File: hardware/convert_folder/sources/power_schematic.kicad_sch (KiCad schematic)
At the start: 31 parts, among them CN1 5-146285-2, CN11 5-146285-2, CN13 4243-0, CN15 JST 2 position header 2.5mm, CN2 4243-0, CN3 4 pin Picoblade, CN7 5-146285-2, CN8 5-146285-2, CN9 5-146285-2, IC1 TPS3780BDBVT, J3 1054500101, J8 87832-1420, J9 87832-1420

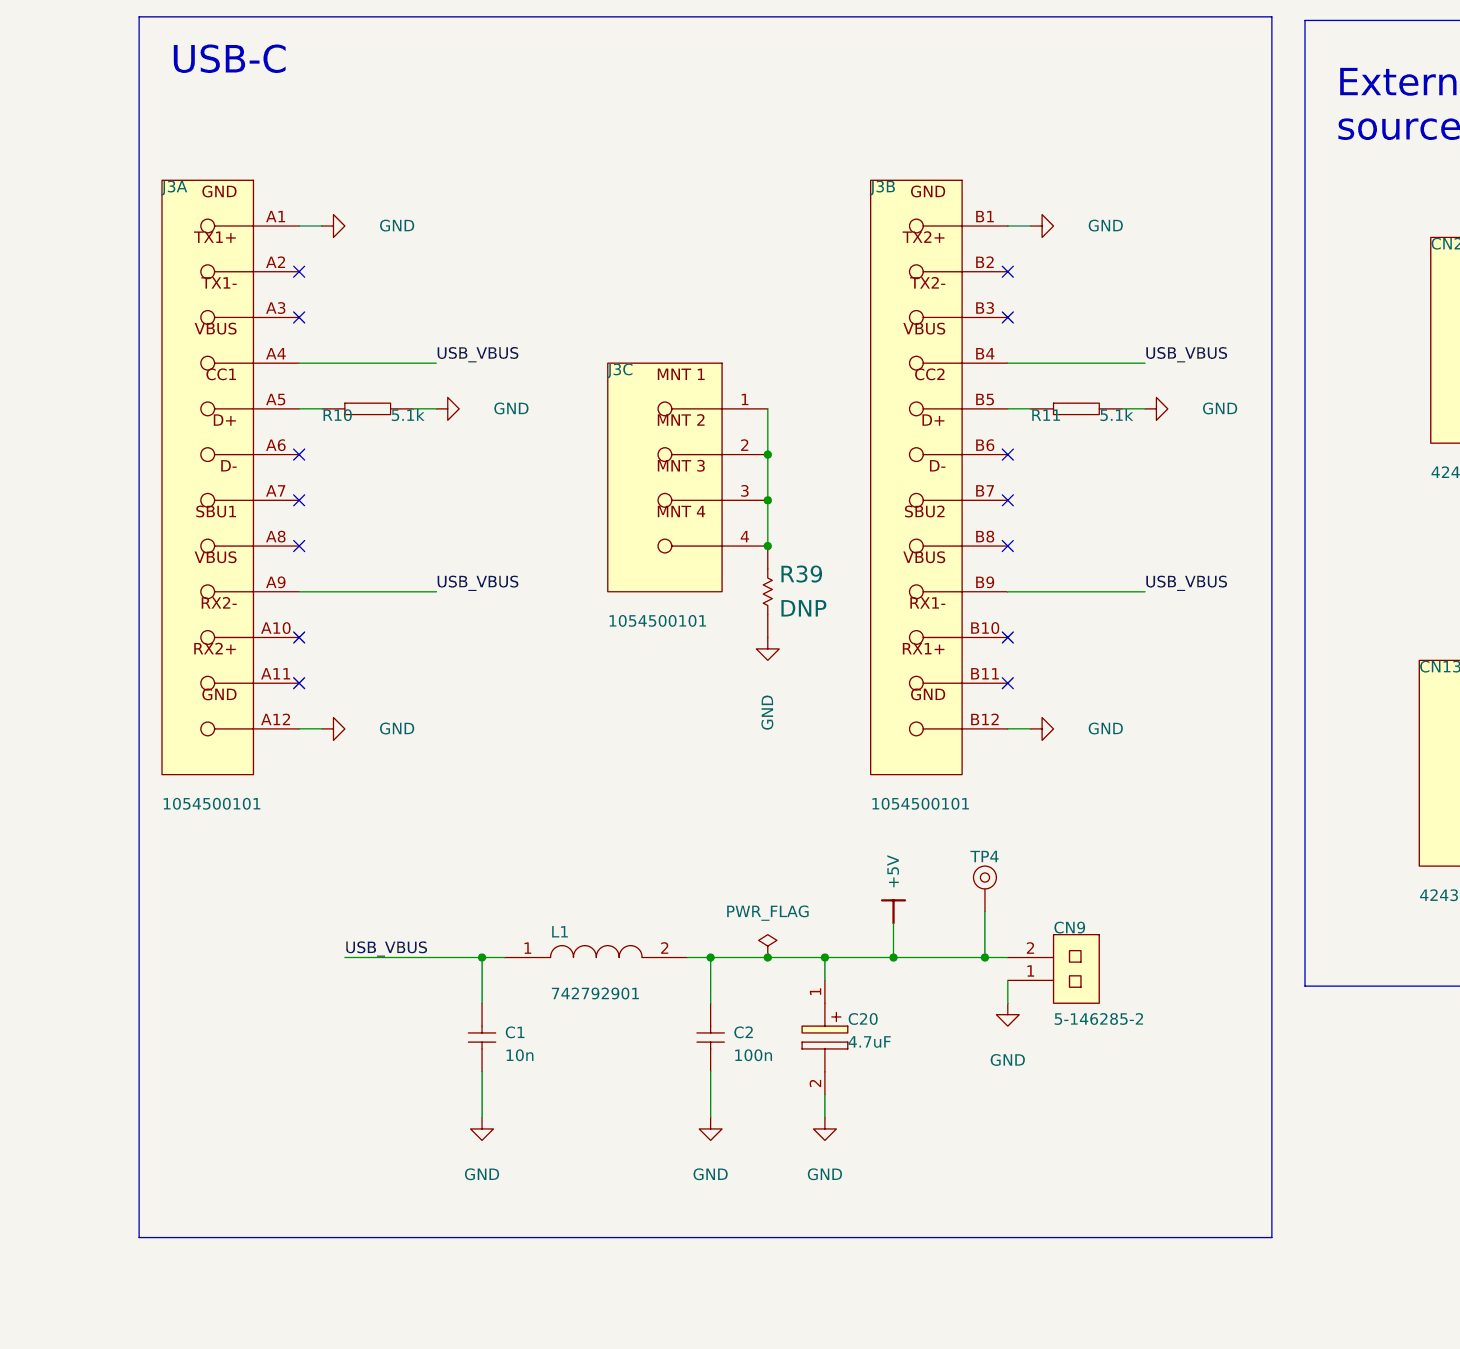
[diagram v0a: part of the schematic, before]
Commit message: chore: add minor modifications do the layout
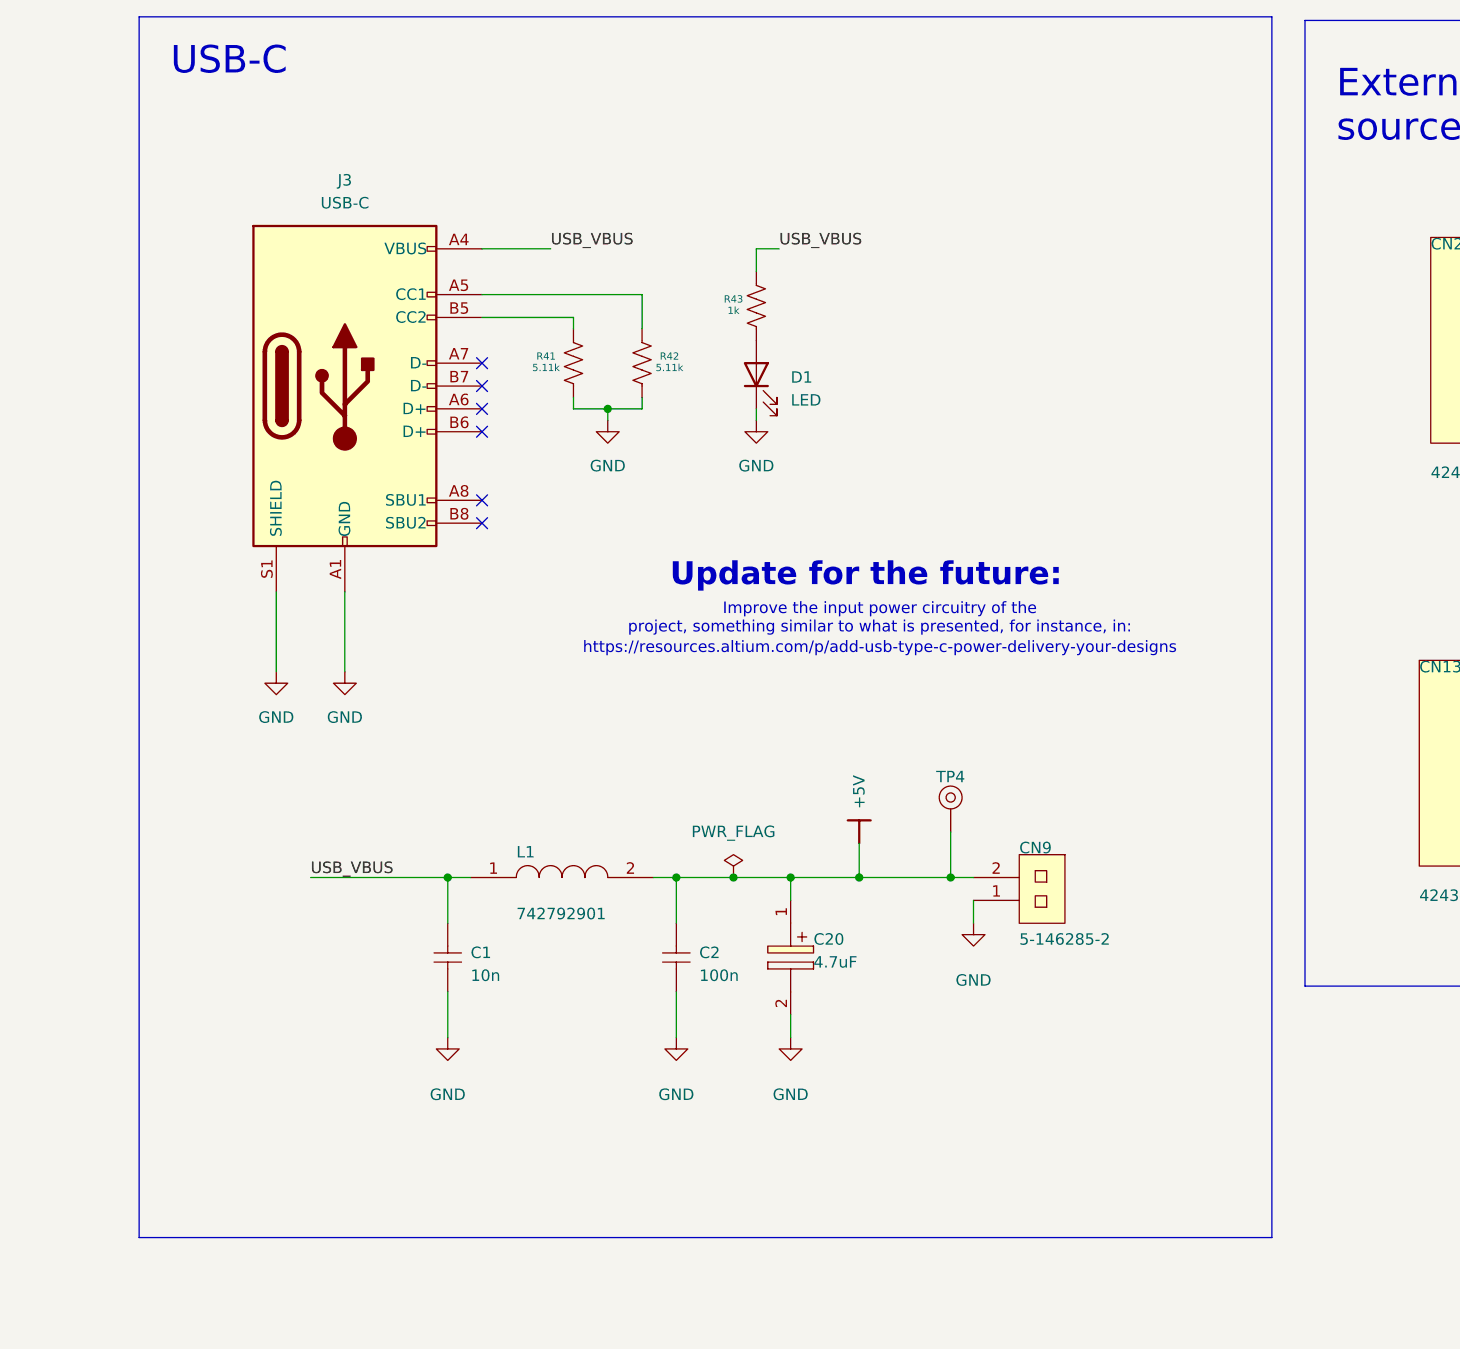
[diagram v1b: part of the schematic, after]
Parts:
- removed J3: 1054500101, altium_import:FP-1054500101-MFG, symbol altium_import:root_0_9808b19ecaf079fb99eed69f0495cd0_Altium Content Vault
- removed R10, R11: RMCF0603FT5K10, altium_import:R0603_MD, symbol altium_import:root_1_RMCF0603FT5K10_Resistor.SchLib
- removed R39: DNP, altium_import:0805, symbol altium_import:RDNP_0805
- added D1: LED, LED_SMD:LED_0603_1608Metric, symbol Device:LED
- added J3: USB-C, altium_import:FP-1054500101-MFG, symbol connectors:USB-C
- added R41, R42: 5.11k, footprints:RES0402, symbol resistors:CRCW04025K11FKED
- added R43: 1k, footprints:RES0603, symbol resistors:CRCW06031K00FKEAHP
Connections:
- net GND: now also D1.1 (K), J3.A1 (GND), J3.A12 (GND), J3.B1 (GND), J3.B12 (GND), J3.S1 (SHIELD), R41.1, R42.1
- net USB_VBUS: now also J3.A4 (VBUS), J3.A9 (VBUS), J3.B4 (VBUS), J3.B9 (VBUS), R43.2
- new net: J3.B5 (CC2), R41.2
- new net: J3.A5 (CC1), R42.2
- new net: D1.2 (A), R43.1
- no-connect marks 14 -> 6
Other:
- note added: "Improve the input power circuitry of the project, something similar to what is presented, for instance, in:"
- note added: "Update for the future:"
- note added: "https://resources.altium.com/p/add-usb-type-c-power-delivery-your-designs"
- moved on the sheet: C1, C2, C20, CN9, L1, TP4

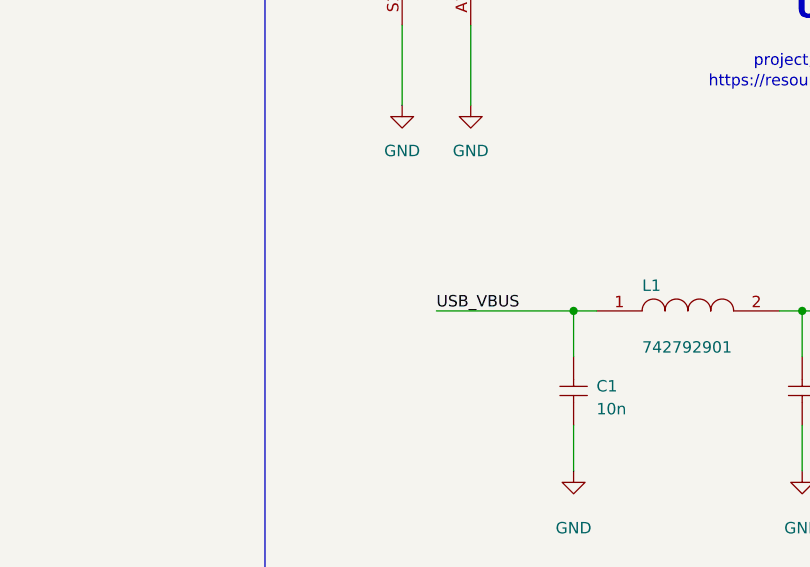
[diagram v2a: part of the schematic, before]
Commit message: fix: improve CAN-related routing and other minor layout-related things
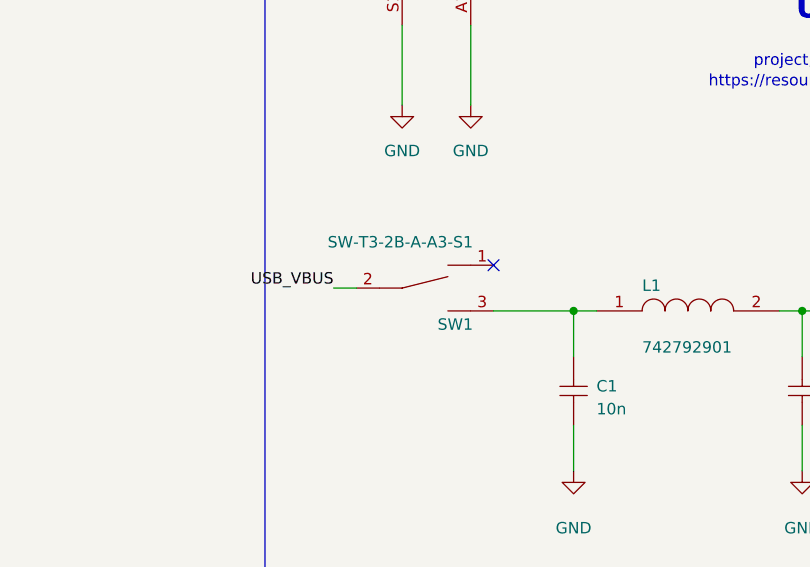
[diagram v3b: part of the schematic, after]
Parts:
- added SW1: SW-T3-2B-A-A3-S1, altium_import:SW-T3-2B-A-A3-S1, symbol altium_import:root_2_SW-T3-2B-A-A3-S1_SW-T3-2B-A-A3-S1.SchLib
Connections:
- net USB_VBUS: now also SW1.2 (COM); no longer C1.1, L1.1
- new net: C1.1, L1.1, SW1.3
- no-connect marks 6 -> 7
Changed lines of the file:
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@@
+	)
+	(no_connect
+		(at 228.6 124.46)
 	)
 	(no_connect
@@
 	(wire
 		(pts
+			(xy 210.82 127) (xy 213.36 127)
+		)
+		(stroke
+			(width 0.381)
+			(type default)
+		)
+	)
+	(wire
+		(pts
 			(xy 36.83 237.49) (xy 54.61 237.49)
 		)
@@
 	(wire
 		(pts
-			(xy 237.49 129.54) (xy 222.25 129.54)
+			(xy 237.49 129.54) (xy 228.6 129.54)
 		)
 		(stroke
@@
 	)
 	(label "USB_VBUS"
-		(at 222.25 129.54 0)
-		(effects
-			(font
-				(size 1.27 1.27)
-			)
-			(justify left bottom)
+		(at 210.82 127 180)
+		(effects
+			(font
+				(size 1.27 1.27)
+			)
+			(justify right bottom)
 		)
 	)
@@
 					(unit 1)
 				)
+			)
+		)
+	)
+	(symbol
+		(lib_id "altium_import:root_2_SW-T3-2B-A-A3-S1_SW-T3-2B-A-A3-S1.SchLib")
+		(at 223.52 127 90)
+		(unit 1)
+		(exclude_from_sim no)
+		(in_bom yes)
+		(on_board yes)
+		(dnp no)
+		(property "Reference" "SW1"
+			(at 226.314 130.302 90)
+			(effects
+				(font
+					(size 1.27 1.27)
+				)
+				(justify left bottom)
+			)
+		)
+		(property "Value" "SW-T3-2B-A-A3-S1"
+			(at 226.314 121.158 90)
+			(effects
+				(font
+					(size 1.27 1.27)
+				)
+				(justify left bottom)
+			)
+		)
+		(property "Footprint" "altium_import:SW-T3-2B-A-A3-S1"
+			(at 223.52 127 0)
+			(effects
+				(font
+					(size 1.27 1.27)
+				)
+				(hide yes)
+			)
+		)
+		(property "Datasheet" ""
+			(at 223.52 127 0)
+			(effects
+				(font
+					(size 1.27 1.27)
+				)
+				(hide yes)
+			)
+		)
+		(property "Description" "SW-T3-2B-A-A3-S1"
+			(at 223.52 127 0)
+			(effects
+				(font
+					(size 1.27 1.27)
+				)
+				(hide yes)
+			)
+		)
+		(pin "2"
+		)
+		(pin "1"
+		)
+		(pin "3"
+		)
+		(instances
+			(project "flatsat_platform_2"
+				(path "/8c88a7e1-4137-48d7-b926-b5e762e3852f/8386d232-e6d5-4b15-8289-83f2ee4d46fe"
+					(reference "SW1")
+					(unit 1)
+				)
